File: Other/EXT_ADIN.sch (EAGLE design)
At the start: 19 parts, among them IC1 TINY45, Q1 IRLU3410, Q2 IRLU3410, Q3 IRLU3410, X2 PW1

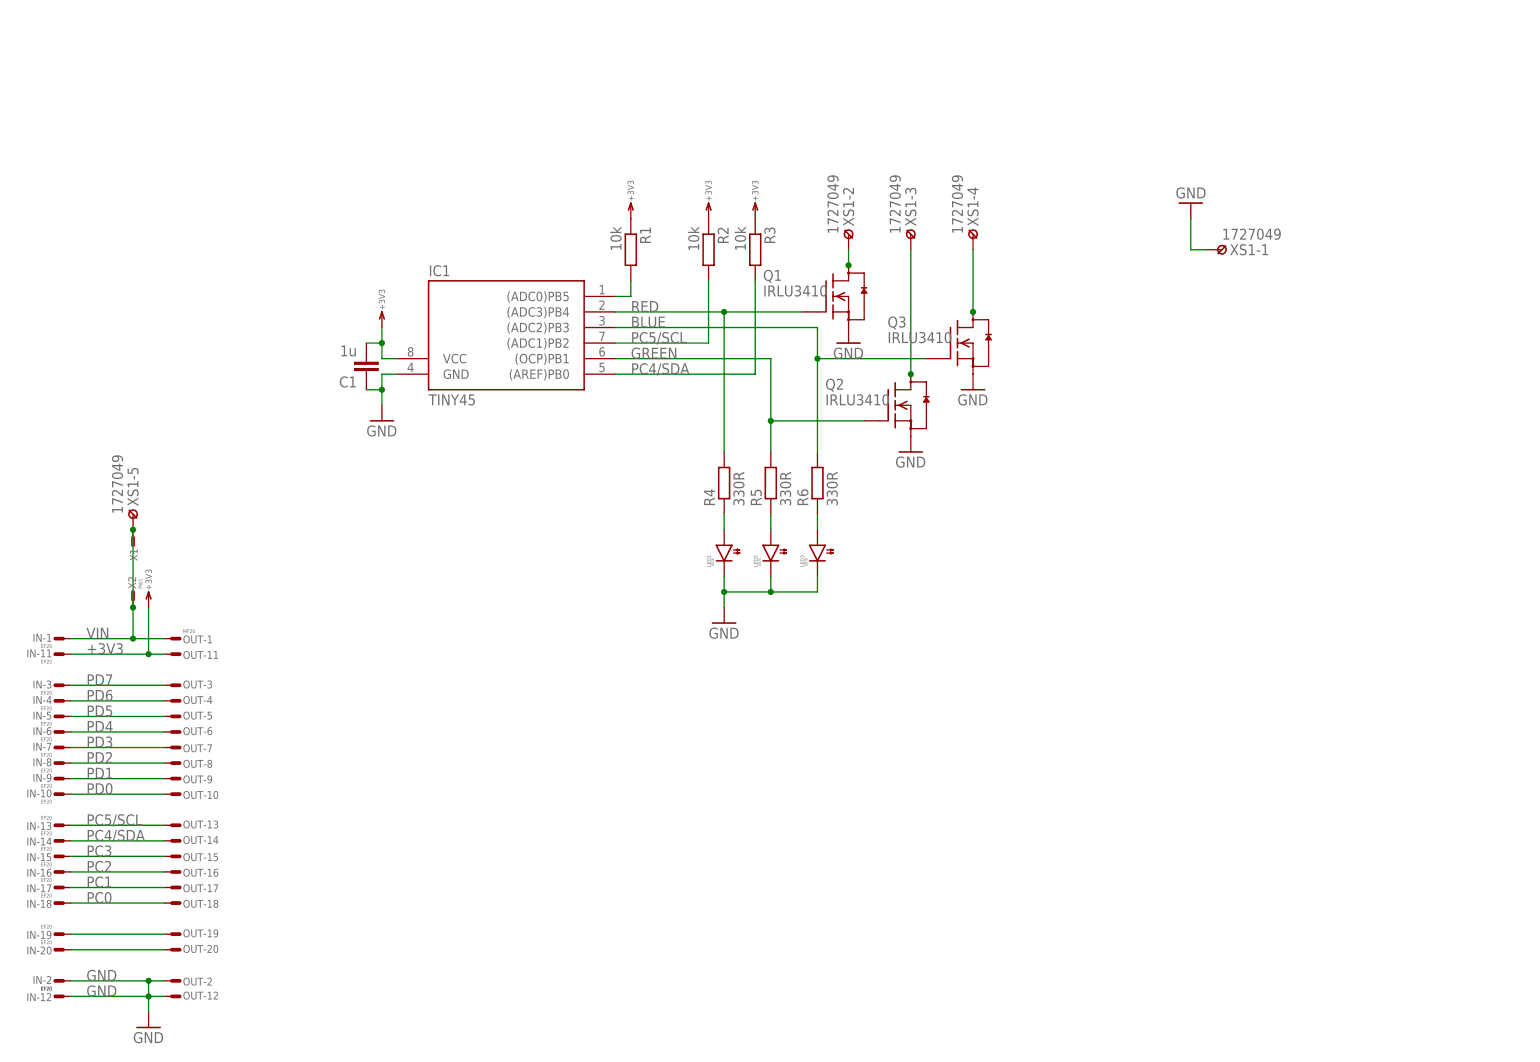
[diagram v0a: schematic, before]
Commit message: Added ...
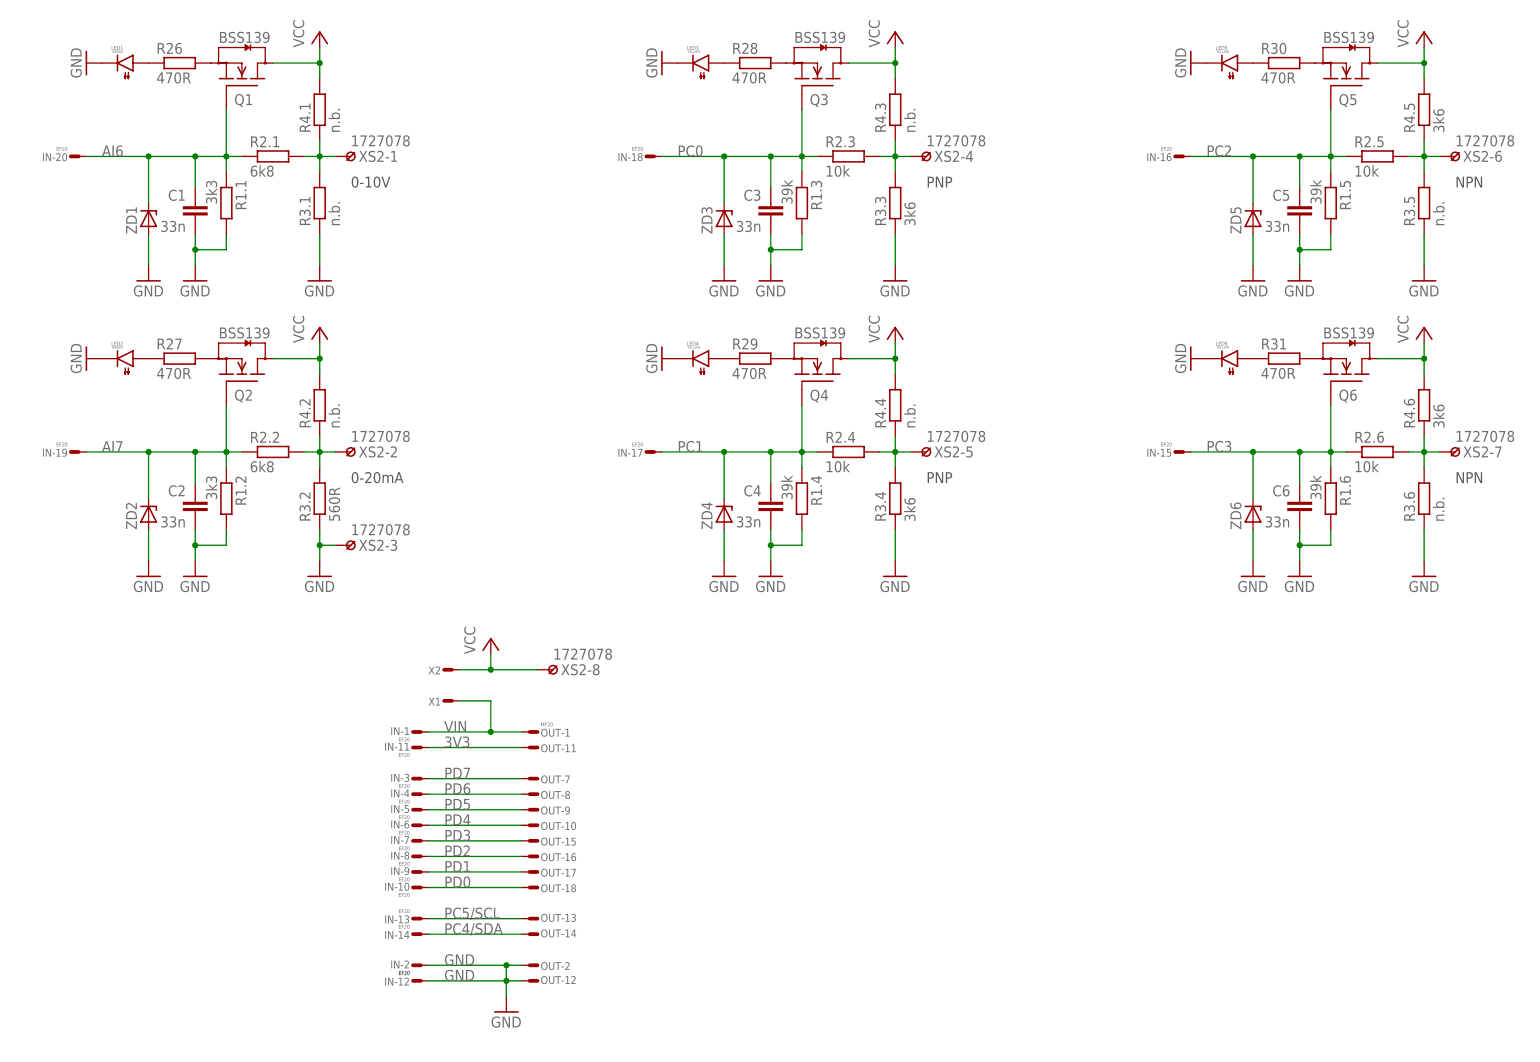
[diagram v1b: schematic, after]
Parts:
- removed IC1: TINY45, atmel:TINY15LS
- removed R1, R2, R3: 10k, RCL:R0603
- removed R4, R5, R6: 330R, RCL:R0603
- removed XS1: 1727049, Conn:1727049
- added C2, C3, C4, C5, C6: 33n, RCL:C1206
- added LED4, LED5, LED6: YELLOW, Optic:LED1206
- added Q4, Q5, Q6: BSS139, Transistor:FET-ND23
- added R1.1, R1.2: 3k3, RCL:R1206
- added R1.3, R1.4, R1.5, R1.6: 39k, RCL:R1206
- added R2.1, R2.2: 6k8, RCL:R1206
- added R2.3, R2.4, R2.5, R2.6: 10k, RCL:R1206
- added R26, R27, R28, R29, R30, R31: 470R, RCL:R1206
- added R3.1, R3.5, R3.6, R4.1, R4.2, R4.3, R4.4: n.b., RCL:R1206
- added R3.2: 560R, RCL:R1206
- added R3.3, R3.4, R4.5, R4.6: 3k6, RCL:R1206
- added XS2: 1727078, Conn:CON8-SS381
- added ZD1, ZD2, ZD3, ZD4, ZD5, ZD6: (no value), Diode:ZDSOD80
- C1: value 1u -> 33n; device RCL:C0603 -> RCL:C1206
- LED1: value LEDR -> GREEN
- LED2: value LEDG -> GREEN
- LED3: value LEDB -> YELLOW
- Q1, Q2, Q3: value IRLU3410 -> BSS139; device Transistor:FET-ND251 -> Transistor:FET-ND23
- X2: value PW1 -> (none)
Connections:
- removed net +3V3: C1.2, IC1.VCC, IN-11.S, OUT-11.S, R1.1, R2.1, R3.1
- removed net BLUE: IC1.(ADC2)PB3, Q3.G, R6.2
- removed net GREEN: IC1.(OCP)PB1, Q2.G, R5.2
- removed net N$7: Q2.D, XS1-3.K
- removed net RED: IC1.(ADC3)PB4, Q1.G, R4.2
- removed net RST: IC1.(ADC0)PB5, R1.2
- new net 3V3: IN-11.S, OUT-11.S
- new net AI6: C1.1, IN-20.S, Q1.G, R1.1.1, R2.1.1, ZD1.C
- new net AI7: C2.1, IN-19.S, Q2.G, R1.2.1, R2.2.1, ZD2.C
- new net N$10: LED2.A, R27.1
- new net N$11: Q2.S, R27.2
- new net N$12: LED3.A, R28.1
- new net N$13: Q3.S, R28.2
- new net N$14: LED4.A, R29.1
- new net N$15: Q4.S, R29.2
- new net N$16: LED5.A, R30.1
- new net N$17: Q5.S, R30.2
- new net N$18: LED6.A, R31.1
- new net N$19: Q6.S, R31.2
- new net N$2: R2.3.2, R3.3.2, R4.3.1, XS2-4.K
- new net VCC: Q1.D, Q2.D, Q3.D, Q4.D, Q5.D, Q6.D, R4.1.2, R4.2.2, R4.3.2, R4.4.2, R4.5.2, R4.6.2, X2.S, XS2-8.K
- net GND: now also C1.2, C2.2, C3.2, C4.2, C5.2, C6.2, LED4.C, LED5.C, LED6.C, R1.1.2, R1.2.2, R1.3.2, R1.4.2, R1.5.2, R1.6.2, R3.1.1, R3.2.1, R3.3.1, R3.4.1, R3.5.1, R3.6.1, XS2-3.K, ZD1.A, ZD2.A, ZD3.A, ZD4.A, ZD5.A, ZD6.A; no longer C1.1, IC1.GND, Q1.S, Q2.S, Q3.S, XS1-1.K
- net N$1: now also R2.2.2, R3.2.2, R4.2.1, XS2-2.K; no longer IN-20.S, OUT-20.S
- net N$3: now also R2.1.2, R3.1.2, R4.1.1, XS2-1.K; no longer IN-19.S, OUT-19.S
- net N$4: now also R2.4.2, R3.4.2, R4.4.1, XS2-5.K; no longer LED1.A, R4.1
- net N$5: now also R2.5.2, R3.5.2, R4.5.1, XS2-6.K; no longer LED2.A, R5.1
- net N$6: now also R2.6.2, R3.6.2, R4.6.1, XS2-7.K; no longer Q1.D, XS1-2.K
- net N$8: now also LED1.A, R26.1; no longer Q3.D, XS1-4.K
- net N$9: now also Q1.S, R26.2; no longer LED3.A, R6.1
- net PC0: now also C3.1, Q3.G, R1.3.1, R2.3.1, ZD3.C; no longer OUT-18.S
- net PC1: now also C4.1, Q4.G, R1.4.1, R2.4.1, ZD4.C; no longer OUT-17.S
- net PC2: now also C5.1, Q5.G, R1.5.1, R2.5.1, ZD5.C; no longer OUT-16.S
- net PC3: now also C6.1, Q6.G, R1.6.1, R2.6.1, ZD6.C; no longer OUT-15.S
- net PC4/SDA: no longer IC1.(AREF)PB0, R3.2
- net PC5/SCL: no longer IC1.(ADC1)PB2, R2.2
- net PD0: now also OUT-18.S; no longer OUT-10.S
- net PD1: now also OUT-17.S; no longer OUT-9.S
- net PD2: now also OUT-16.S; no longer OUT-8.S
- net PD3: now also OUT-15.S; no longer OUT-7.S
- net PD4: now also OUT-10.S; no longer OUT-6.S
- net PD5: now also OUT-9.S; no longer OUT-5.S
- net PD6: now also OUT-8.S; no longer OUT-4.S
- net PD7: now also OUT-7.S; no longer OUT-3.S
- net VIN: no longer X2.S, XS1-5.K
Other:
- note added: "0-10V"
- note added: "0-20mA"
- note added: "NPN"
- note added: "PNP"
- moved on the sheet: C1, IN-1, IN-10, IN-11, IN-12, IN-13, IN-14, IN-15, IN-16, IN-17, IN-18, IN-19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
